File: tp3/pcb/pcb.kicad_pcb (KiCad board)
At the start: 2 copper layers, 55.5 x 50 mm, 21 parts, among them J1 Screw_Terminal_01x02, J2 Screw_Terminal_01x03, J3 Conn_01x02_Pin, U1 TL084

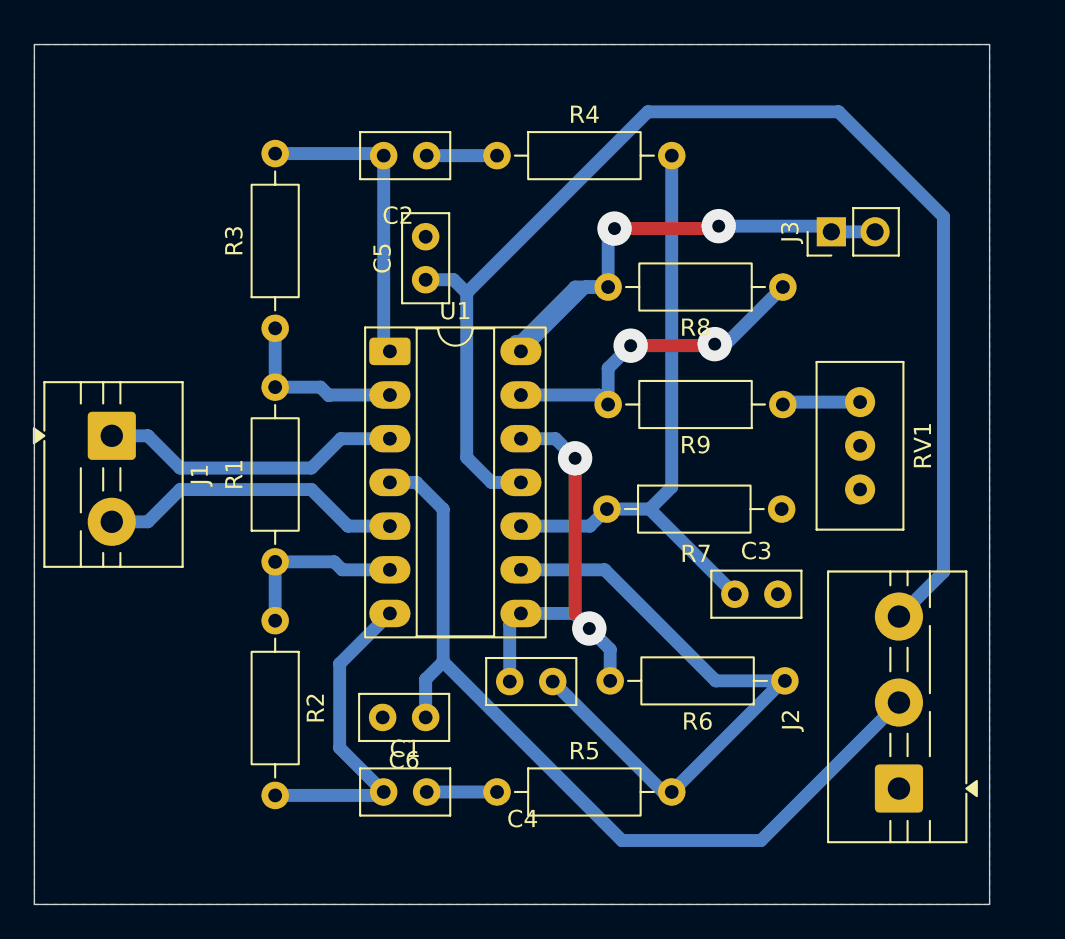
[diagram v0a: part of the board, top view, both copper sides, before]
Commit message: rayo chunkificador
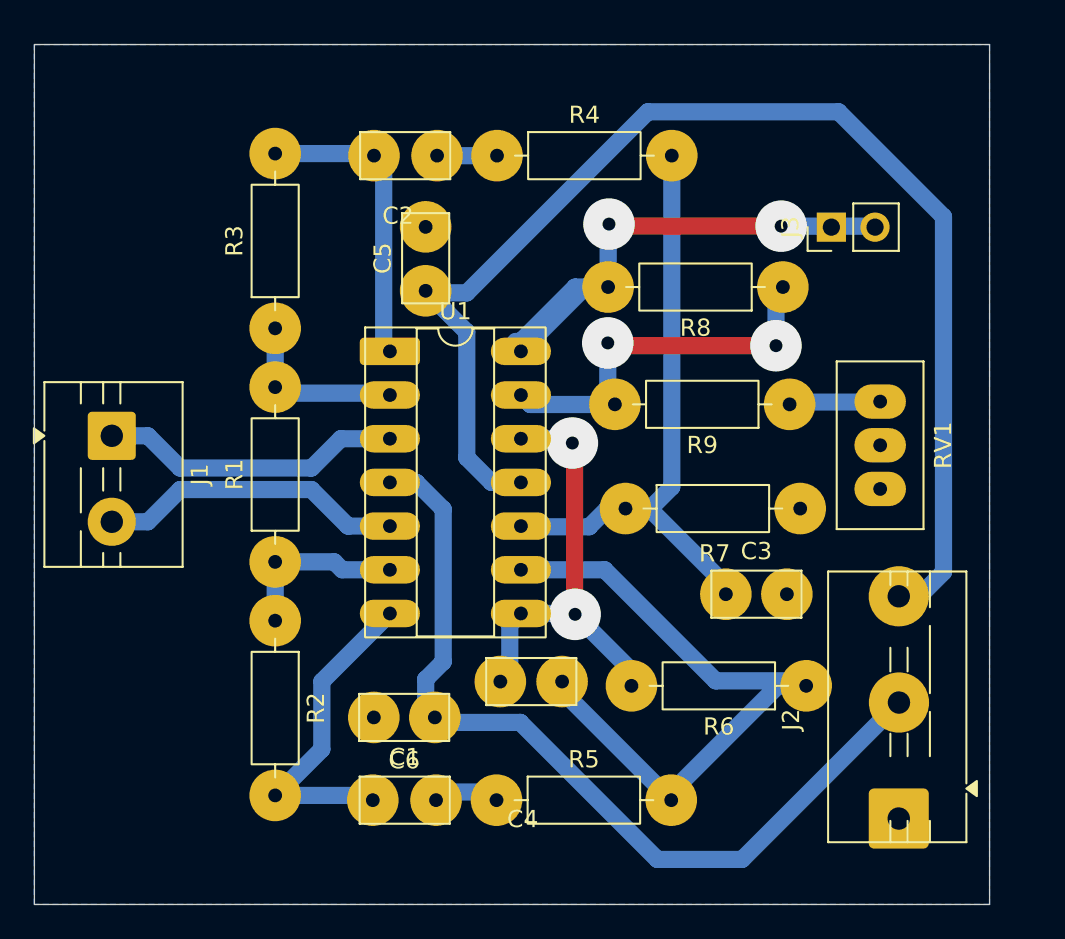
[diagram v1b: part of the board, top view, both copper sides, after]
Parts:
- moved R6 1.27 mm to (150.9, 145.3)
- moved RV1 1.17 mm to (155.2, 133.8)
- moved R7 1.08 mm to (140.4, 135.0)
- moved C1 0.48 mm to (126.3, 151.9)
- moved R5 0.48 mm to (132.9, 151.9)
- moved R9 0.39 mm to (149.9, 128.9)
- moved J3 0.27 mm to (152.3, 118.6)
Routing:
- net Net-(U1D--): track 19.5 -> 22.9 mm
- net /Vo_N: track 36.9 -> 39.3 mm
- net /V_Processed: track 24.8 -> 26.0 mm
- net -15V: track 75.0 -> 76.1 mm
